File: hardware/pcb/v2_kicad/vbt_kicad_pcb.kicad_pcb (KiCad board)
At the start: 2 copper layers, 70 x 50 mm, 22 parts, among them J1 Conn_01x03, J2 Conn_01x05, J3 Conn_01x04, J4 Conn_01x04, J8 Conn_01x04, SW1 SW_Push, SW2 SW_Push, U1 ESP32-WROOM-32E

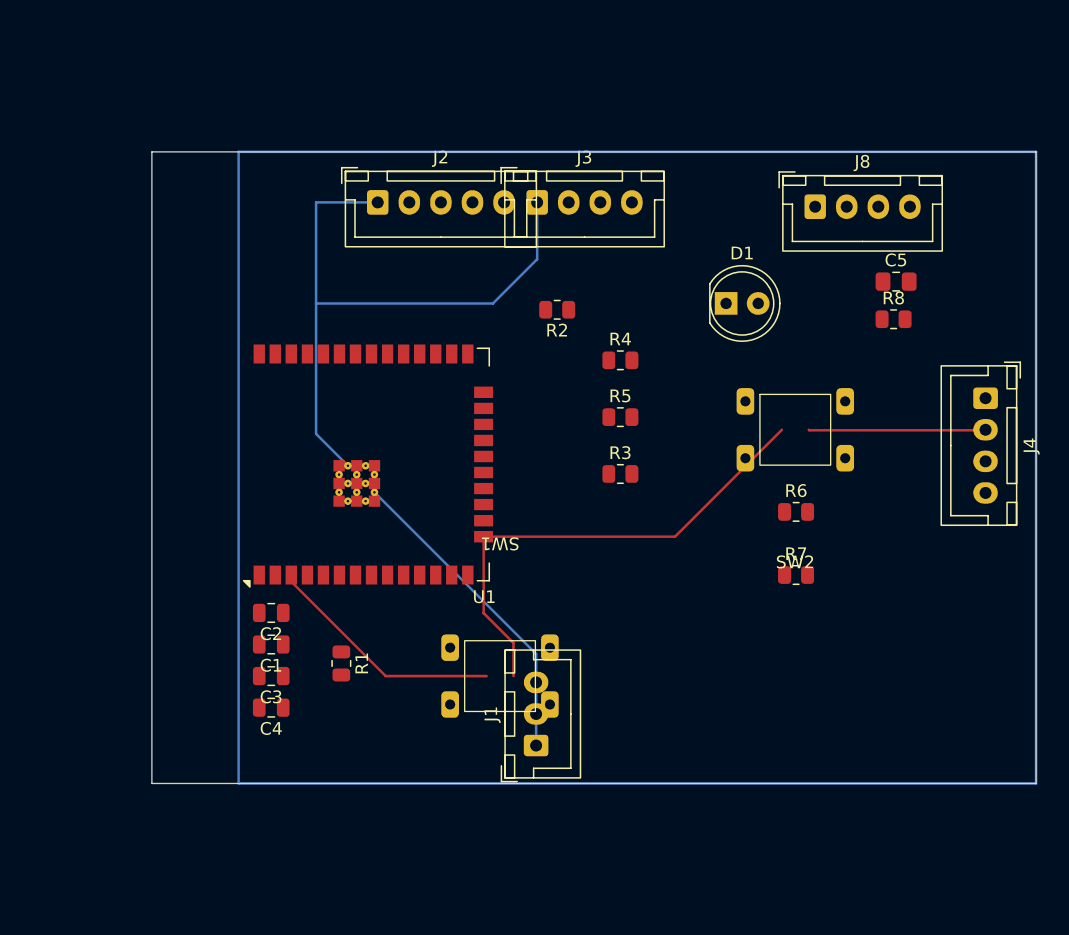
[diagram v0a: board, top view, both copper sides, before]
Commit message: updated pcb layout
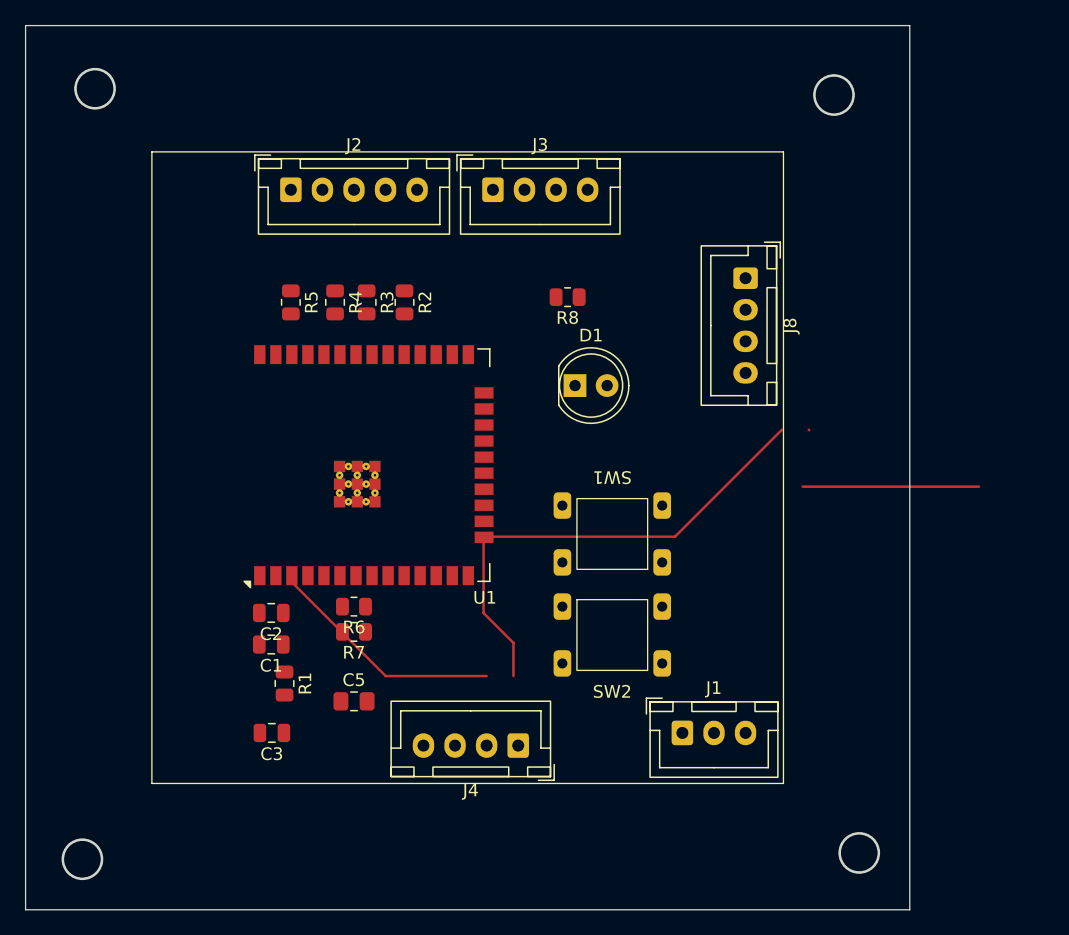
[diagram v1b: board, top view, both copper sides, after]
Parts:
- removed C4: 1 µF, Capacitor_SMD:C_0805_2012Metric
- J1: value Conn_01x03 -> Serial Connector
- J2: value Conn_01x05 -> Rotary Encoder
- J3: value Conn_01x04 -> I2C Display
- J4: value Conn_01x04 -> Power Connector
- J8: value Conn_01x04 -> I2C Magnet Sensor
- moved C5 54.3 mm to (125.0, 94.5)
- moved J4 46.1 mm to (138.0, 98.0), turned to 180 degrees
- moved R6 35.8 mm to (125.0, 87.0), turned to 180 degrees
- moved R7 35.3 mm to (125.0, 89.0), turned to 180 degrees
- moved R5 27.6 mm to (120.0, 62.9), turned to -90 degrees
- moved R8 25.9 mm to (141.9, 62.5), turned to 180 degrees
- moved R3 24.3 mm to (126.0, 62.9), turned to -90 degrees
- moved R4 23.0 mm to (123.5, 62.9), turned to -90 degrees
- moved SW2 21.8 mm to (145.4, 89.2)
- moved SW1 14.3 mm to (145.4, 81.2)
- moved D1 13.6 mm to (142.5, 69.5)
- moved R2 12.1 mm to (129.0, 62.9), turned to -90 degrees
- moved J1 11.6 mm to (151.0, 97.0), turned to 0 degrees
- moved J8 7.90 mm to (156.0, 61.0), turned to -90 degrees
- moved J2 6.95 mm to (120.0, 54.0)
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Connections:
- C1 pad 2: Net-(J1-Pin_3) -> GND
- C2 pad 2: Net-(J1-Pin_3) -> GND
- C3 pad 2: Net-(J1-Pin_3) -> GND
- C5 pad 2: Net-(J1-Pin_3) -> GND
- J1 pad 3: Net-(J1-Pin_3) -> GND
- R7 pad 1: Net-(J1-Pin_3) -> GND
- SW1 pad 1: Net-(J1-Pin_3) -> GND
- SW2 pad 1: Net-(J1-Pin_3) -> GND
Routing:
- net GND: track 128.7 -> 39.1 mm
- net /ESP_RX: track 0.00 -> 14.0 mm
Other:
- board size 70 x 50 mm -> 70 x 70 mm
